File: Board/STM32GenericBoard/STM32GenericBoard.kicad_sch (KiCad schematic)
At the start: 14 parts, among them SW1 SW_Push, U2 ICM-45686, U3 SN65HVD230, U4 AMS1117-3.3, U5 STM32H743VGTx

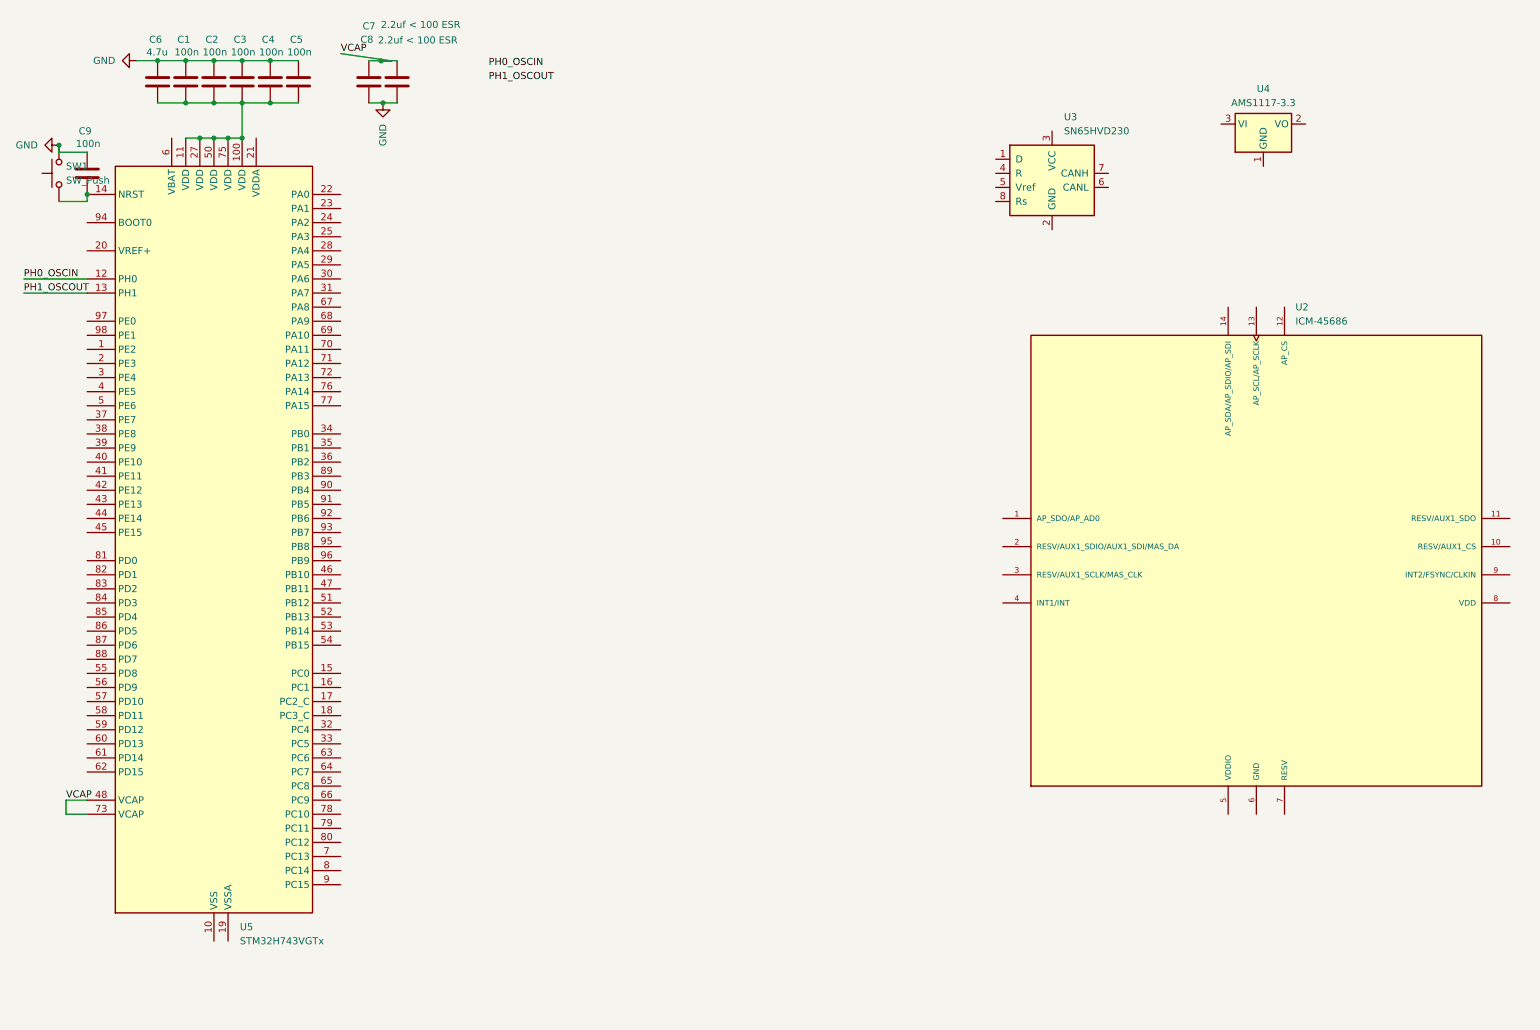
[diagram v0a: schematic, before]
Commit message: Save board
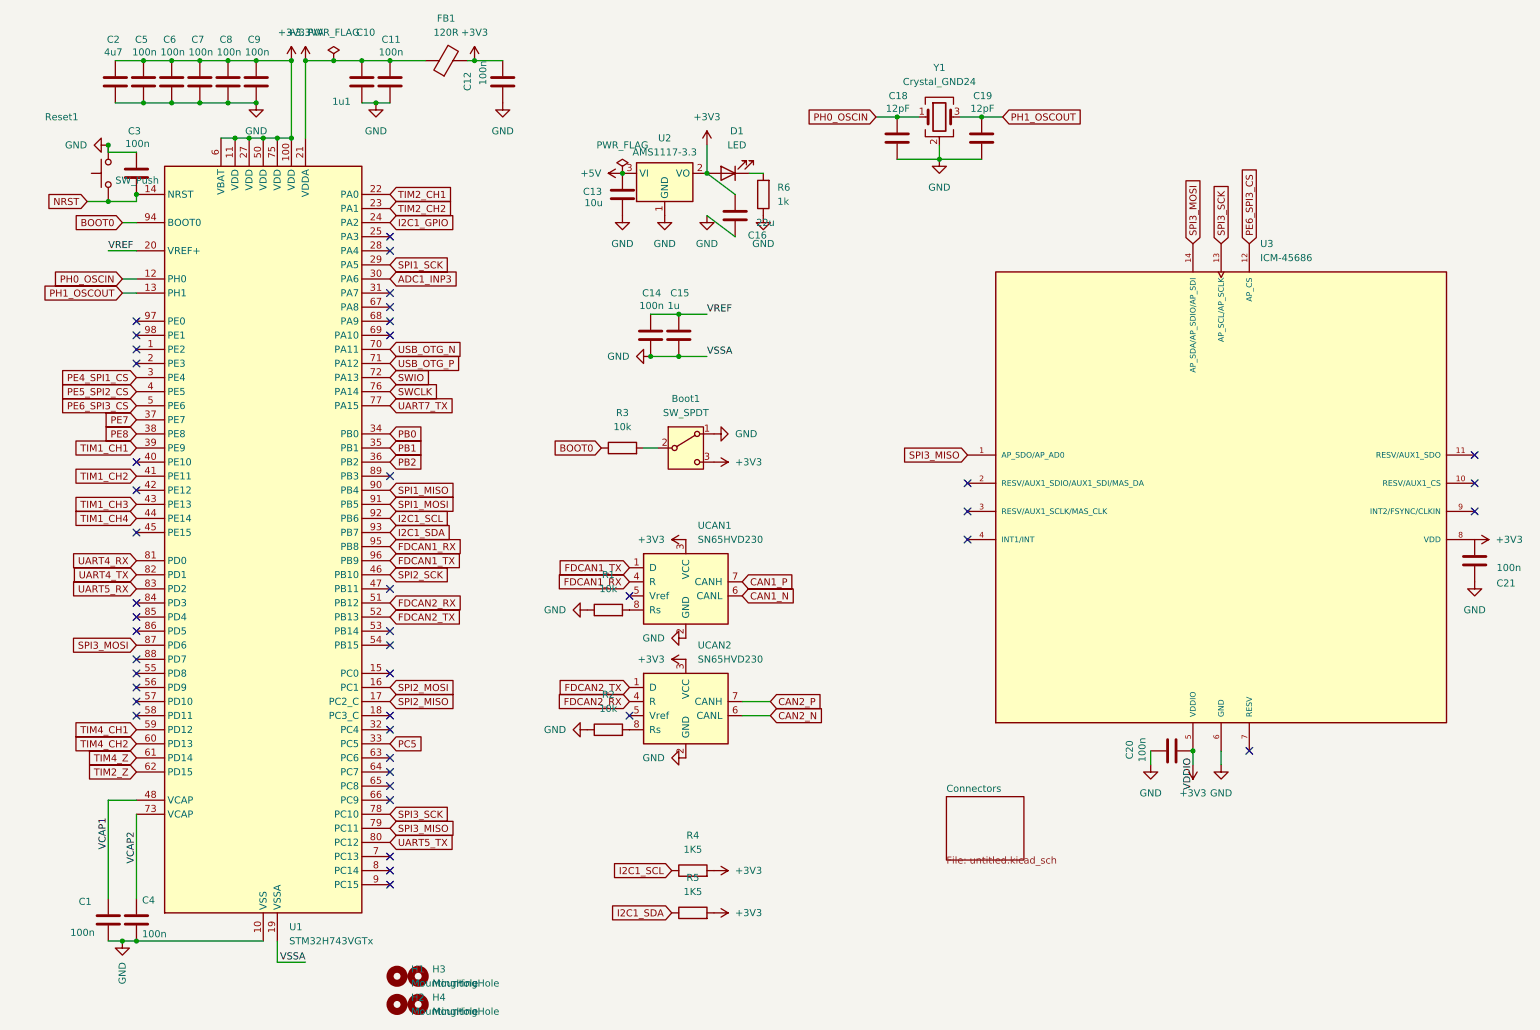
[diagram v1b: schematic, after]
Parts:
- added Boot1: SW_SPDT, Button_Switch_SMD:SW_SPDT_PCM12, symbol Switch:SW_SPDT
- added C10: 1u1, Capacitor_SMD:C_0603_1608Metric_Pad1.08x0.95mm_HandSolder, symbol Device:C
- added C11, C12, C14, C20, C21: 100n, Capacitor_SMD:C_0402_1005Metric_Pad0.74x0.62mm_HandSolder, symbol Device:C
- added C13: 10u, Capacitor_SMD:C_0603_1608Metric_Pad1.08x0.95mm_HandSolder, symbol Device:C
- added C15: 1u, Capacitor_SMD:C_0603_1608Metric_Pad1.08x0.95mm_HandSolder, symbol Device:C
- added C16: 22u, Capacitor_SMD:C_0805_2012Metric_Pad1.18x1.45mm_HandSolder, symbol Device:C
- added C18, C19: 12pF, Capacitor_SMD:C_0402_1005Metric_Pad0.74x0.62mm_HandSolder, symbol Device:C
- added D1: LED, LED_SMD:LED_0805_2012Metric_Pad1.15x1.40mm_HandSolder, symbol Device:LED
- added FB1: 120R, Inductor_SMD:L_0805_2012Metric_Pad1.05x1.20mm_HandSolder, symbol Device:FerriteBead
- added H1, H2, H3, H4: MountingHole, MountingHole:MountingHole_2.2mm_M2, symbol Mechanical:MountingHole
- added R1, R2, R3: 10k, Resistor_SMD:R_0402_1005Metric_Pad0.72x0.64mm_HandSolder, symbol Device:R
- added R4, R5: 1K5, Resistor_SMD:R_0402_1005Metric_Pad0.72x0.64mm_HandSolder, symbol Device:R
- added R6: 1k, Resistor_SMD:R_0402_1005Metric_Pad0.72x0.64mm_HandSolder, symbol Device:R
- added UCAN2: SN65HVD230, Package_SO:SOIC-8_3.9x4.9mm_P1.27mm, symbol Interface_CAN_LIN:SN65HVD230
- added Y1: Crystal_GND24, Crystal:Crystal_SMD_2520-4Pin_2.5x2.0mm, symbol Device:Crystal_GND24
- C1: renamed from C8; value 2.2uf < 100 ESR -> 100n; footprint (none) -> Capacitor_SMD:C_0402_1005Metric_Pad0.74x0.62mm_HandSolder
- C2: renamed from C6; value 4.7u -> 4u7; footprint (none) -> Capacitor_SMD:C_0603_1608Metric_Pad1.08x0.95mm_HandSolder
- C3: renamed from C9; footprint (none) -> Capacitor_SMD:C_0402_1005Metric_Pad0.74x0.62mm_HandSolder
- C4: renamed from C7; value 2.2uf < 100 ESR -> 100n; footprint (none) -> Capacitor_SMD:C_0402_1005Metric_Pad0.74x0.62mm_HandSolder
- C5: renamed from C1; footprint (none) -> Capacitor_SMD:C_0402_1005Metric_Pad0.74x0.62mm_HandSolder
- C6: renamed from C2; footprint (none) -> Capacitor_SMD:C_0402_1005Metric_Pad0.74x0.62mm_HandSolder
- C7: renamed from C3; footprint (none) -> Capacitor_SMD:C_0402_1005Metric_Pad0.74x0.62mm_HandSolder
- C8: renamed from C4; footprint (none) -> Capacitor_SMD:C_0402_1005Metric_Pad0.74x0.62mm_HandSolder
- C9: renamed from C5; footprint (none) -> Capacitor_SMD:C_0402_1005Metric_Pad0.74x0.62mm_HandSolder
- Reset1: renamed from SW1; footprint (none) -> Button_Switch_SMD:SW_Push_1P1T_NO_Vertical_Wuerth_434133025816
- renumbered U5 to U1, U4 to U2, U2 to U3, U3 to UCAN1
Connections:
- net GND: now also C2.2, C5.2, C6.2, C7.2, C8.2, C9.2, U1.10 (VSS), U1.19 (VSSA), U1.26 (VSS), U1.49 (VSS), U1.74 (VSS), U1.99 (VSS), U2.1 (GND), U3.6 (GND), UCAN1.2 (GND), Boot1.1 (A), C10.2, C11.2, C12.1, C13.2, C14.2, C15.2, C16.2, C18.2, C19.2, C20.1, C21.1, R1.1, R2.1, R6.1, UCAN2.2 (GND), Y1.2 (G), Y1.4 (G); no longer C2.1, C5.1, C6.1, C7.1, C8.1, C9.1
- net PH0_OSCIN: now also C18.1, Y1.1
- net PH1_OSCOUT: now also C19.1, Y1.3
- net NRST: now reaches C3.2, Reset1.1, U1.14 (NRST)
- net SPI3_MISO: now reaches U3.1 (AP_SDO/AP_AD0)
- net SPI3_MISO: now also U1.79 (PC11)
- net PE6_SPI3_CS: now reaches U3.12 (AP_CS)
- net PE6_SPI3_CS: now also U1.5 (PE6)
- net SPI3_SCK: now reaches U3.13 (AP_SCL/AP_SCLK)
- net SPI3_SCK: now also U1.78 (PC10)
- net SPI3_MOSI: now reaches U3.14 (AP_SDA/AP_SDIO/AP_SDI)
- net SPI3_MOSI: now also U1.87 (PD6)
- net +3V3: now reaches U3.5 (VDDIO)
- net +3V3: now also C2.1, C5.1, C6.1, C7.1, C8.1, C9.1, U1.100 (VDD), U1.11 (VDD), U1.27 (VDD), U1.50 (VDD), U1.6 (VBAT), U1.75 (VDD), U2.2 (VO), U3.8 (VDD), UCAN1.3 (VCC), Boot1.3 (C), C12.2, C16.1, C20.2, C21.2, D1.2 (A), FB1.2, R4.2, R5.2, UCAN2.3 (VCC)
- net SPI2_MOSI: now reaches U1.16 (PC1)
- net SPI2_MISO: now reaches U1.17 (PC2_C)
- net VREF: now reaches U1.20 (VREF+)
- net VREF: now also C14.1, C15.1
- net +3.3VA: now reaches U1.21 (VDDA)
- net +3.3VA: now also C10.1, C11.1, FB1.1
- net TIM2_CH1: now reaches U1.22 (PA0)
- net TIM2_CH2: now reaches U1.23 (PA1)
- net I2C1_GPIO: now reaches U1.24 (PA2)
- net SPI1_SCK: now reaches U1.29 (PA5)
- net PE4_SPI1_CS: now reaches U1.3 (PE4)
- net ADC1_INP3: now reaches U1.30 (PA6)
- net PC5: now reaches U1.33 (PC5)
- net PB0: now reaches U1.34 (PB0)
- net PB1: now reaches U1.35 (PB1)
- net PB2: now reaches U1.36 (PB2)
- net PE7: now reaches U1.37 (PE7)
- net PE8: now reaches U1.38 (PE8)
- net TIM1_CH1: now reaches U1.39 (PE9)
- net PE5_SPI2_CS: now reaches U1.4 (PE5)
- net TIM1_CH2: now reaches U1.41 (PE11)
- net TIM1_CH3: now reaches U1.43 (PE13)
- net TIM1_CH4: now reaches U1.44 (PE14)
- net SPI2_SCK: now reaches U1.46 (PB10)
- net FDCAN2_RX: now reaches U1.51 (PB12)
- net FDCAN2_RX: now also UCAN2.4 (R)
- net FDCAN2_TX: now reaches U1.52 (PB13)
- net FDCAN2_TX: now also UCAN2.1 (D)
- net TIM4_CH1: now reaches U1.59 (PD12)
- net TIM4_CH2: now reaches U1.60 (PD13)
- net TIM4_Z: now reaches U1.61 (PD14)
- net TIM2_Z: now reaches U1.62 (PD15)
- net USB_OTG_N: now reaches U1.70 (PA11)
- net USB_OTG_P: now reaches U1.71 (PA12)
- net SWIO: now reaches U1.72 (PA13)
- net SWCLK: now reaches U1.76 (PA14)
- net UART7_TX: now reaches U1.77 (PA15)
- net UART5_TX: now reaches U1.80 (PC12)
- net UART4_RX: now reaches U1.81 (PD0)
- net UART4_TX: now reaches U1.82 (PD1)
- net UART5_RX: now reaches U1.83 (PD2)
- net SPI1_MISO: now reaches U1.90 (PB4)
- net SPI1_MOSI: now reaches U1.91 (PB5)
- net I2C1_SCL: now reaches U1.92 (PB6)
- net I2C1_SCL: now also R4.1
- net I2C1_SDA: now reaches U1.93 (PB7)
- net I2C1_SDA: now also R5.1
- net BOOT0: now reaches U1.94 (BOOT0)
- net BOOT0: now also R3.1
- net FDCAN1_RX: now reaches U1.95 (PB8)
- net FDCAN1_RX: now also UCAN1.4 (R)
- net FDCAN1_TX: now reaches U1.96 (PB9)
- net FDCAN1_TX: now also UCAN1.1 (D)
- net CAN1_N: now reaches UCAN1.6 (CANL)
- net CAN1_P: now reaches UCAN1.7 (CANH)
- net at UCAN1.8 (Rs): now also R1.2
- net +5V: now reaches U2.3 (VI)
- net +5V: now also C13.1
- net VCAP renamed VCAP1
- net VCAP1: no longer C4.1, U1.73 (VCAP)
- new net: D1.1 (K), R6.2
- new net: R2.2, UCAN2.8 (Rs)
- new net: Boot1.2 (B), R3.2
- new net CAN2_N: UCAN2.6 (CANL)
- new net CAN2_P: UCAN2.7 (CANH)
- new net VCAP2: C4.1, U1.73 (VCAP)
- no-connect marks 0 -> 44
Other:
- added sheet Connectors (untitled.kicad_sch)
- moved on the sheet: C1, C2, C3, C4, C5, C6, C7, C8, C9, Reset1, U1, U2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
